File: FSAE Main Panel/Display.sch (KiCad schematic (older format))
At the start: 80 parts, among them U501 TLC6C598, U502 TLC6C5816, U503 TLC6C5816, U504 TLC6C5816

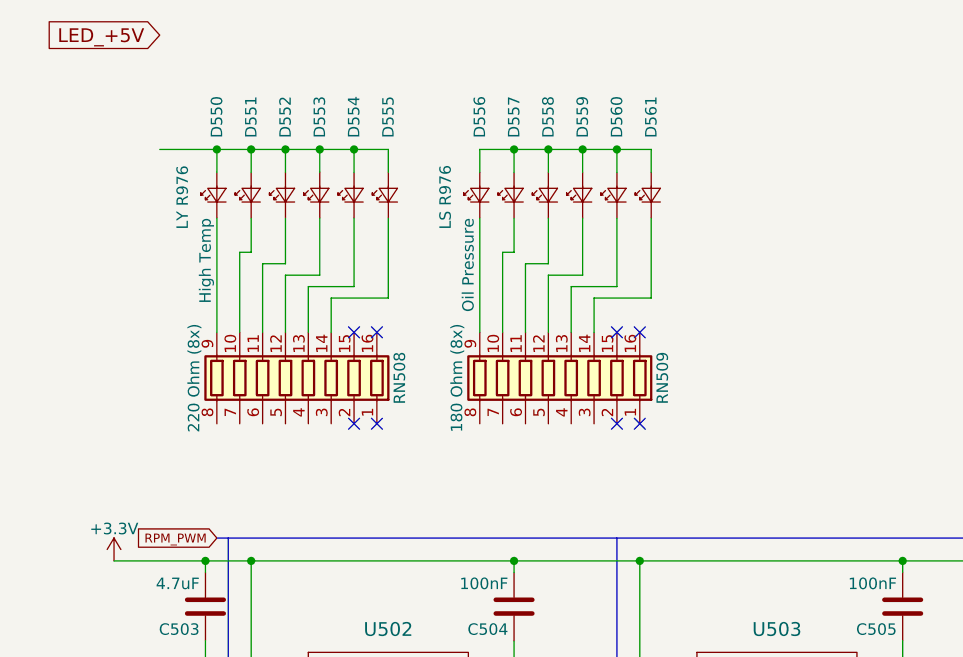
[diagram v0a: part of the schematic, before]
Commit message: Updated PCB
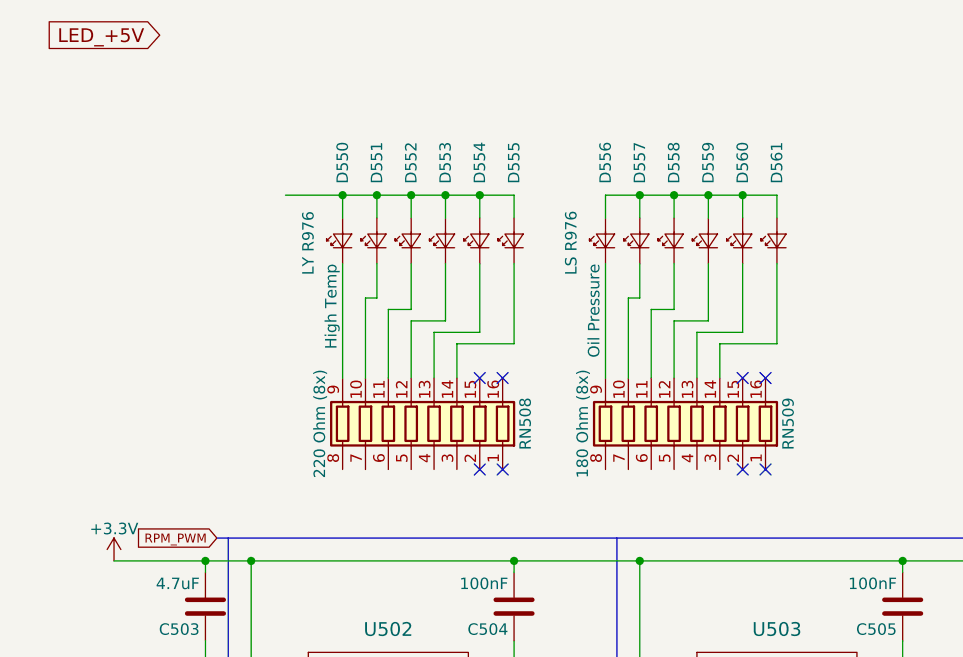
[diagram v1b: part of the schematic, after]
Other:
- moved on the sheet: D550, D551, D552, D553, D554, D555, D556, D557, D558, D559, D560, D561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
